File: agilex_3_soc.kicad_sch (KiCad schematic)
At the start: 11 parts, among them J1 Conn_01x14, J2 Conn_02x03_Odd_Even, J3 Conn_02x19_Odd_Even, J4 Conn_01x03, J5 Conn_01x03, J6 Micro_SD_Card, J7 8P8C_LED_Shielded, U1 IS43LQ32256A-062BLI, U2 ADS7886xxDBV, U3 CD4051B, Y1 ASDMB-25MHz

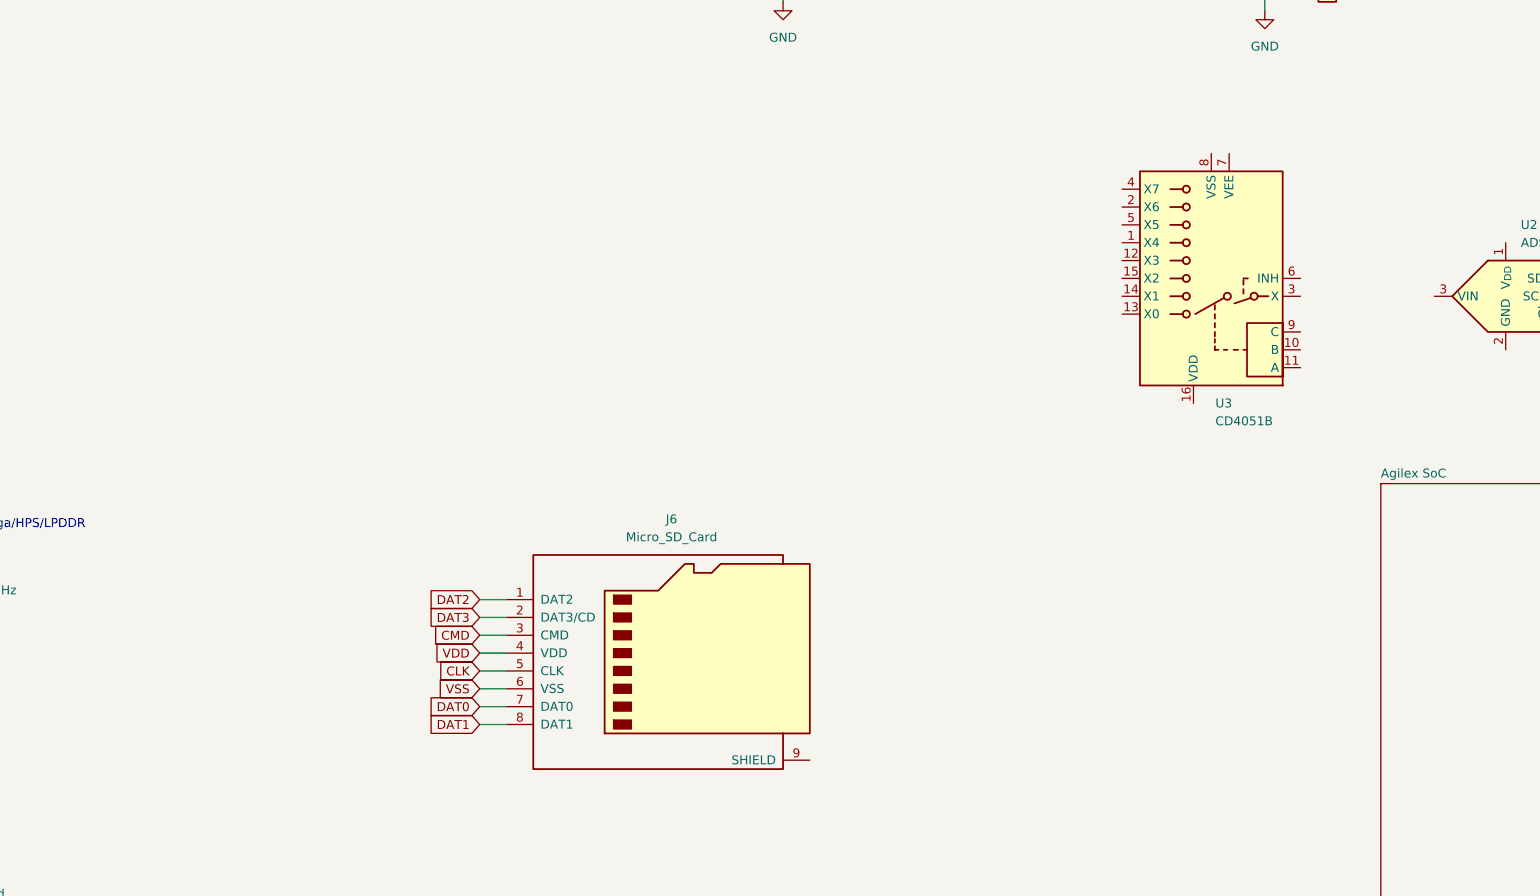
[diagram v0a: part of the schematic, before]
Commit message: start creating schematic symbol for agilex 5
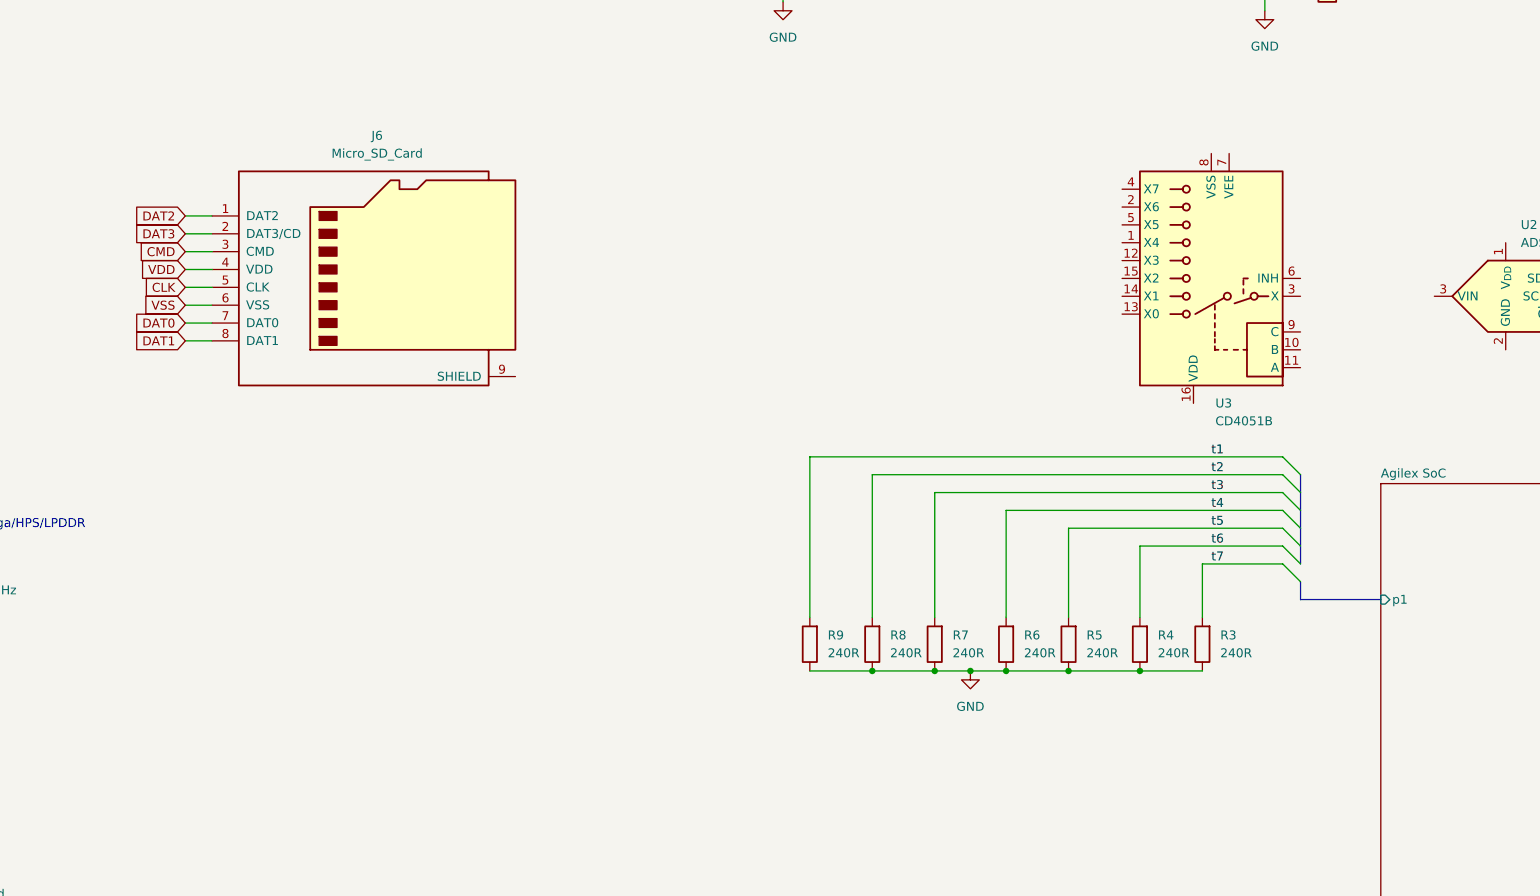
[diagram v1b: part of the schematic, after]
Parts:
- added R3, R4, R5, R6, R7, R8, R9: 240R, Capacitor_SMD:C_0402_1005Metric, symbol Device:R
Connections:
- net GND: now also R3.1, R4.1, R5.1, R6.1, R7.1, R8.1, R9.1
- new net t1: R9.2
- new net t2: R8.2
- new net t3: R7.2
- new net t4: R6.2
- new net t5: R5.2
- new net t6: R4.2
- new net t7: R3.2
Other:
- sheet Agilex SoC ports: added p1; removed none
- moved on the sheet: J6
